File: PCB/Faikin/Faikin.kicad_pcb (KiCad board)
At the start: 2 copper layers, 70 x 70 mm, 31 parts, among them J1 1x5, J2 TC2030-USB-NL-DS, J3 Reset, Q1 BSS138PS, U3 MD8942, U4 ESP32-S3-MINI-1

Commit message: PCB Update
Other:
- board text removed: "TC2030"

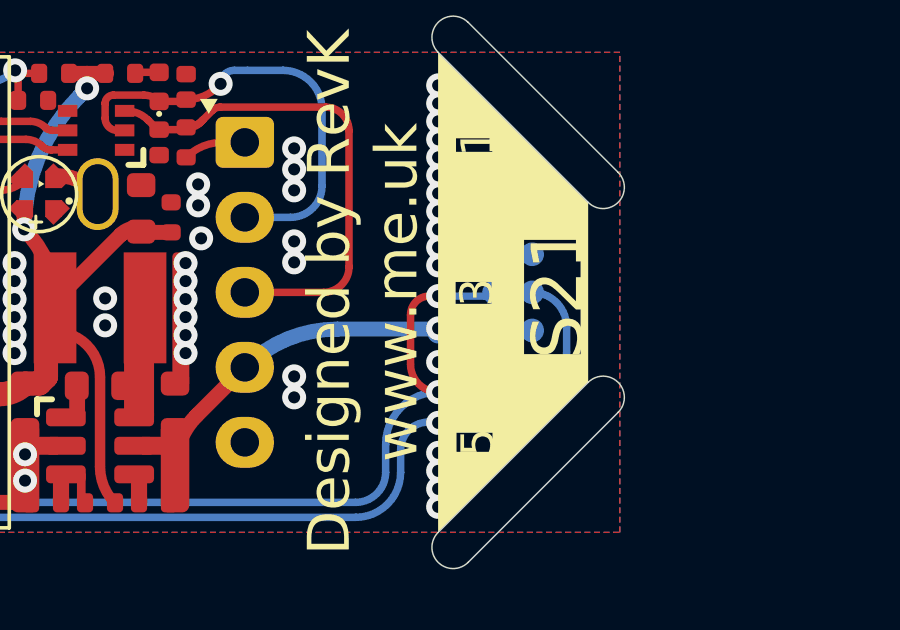
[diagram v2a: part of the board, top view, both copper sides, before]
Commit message: Library update
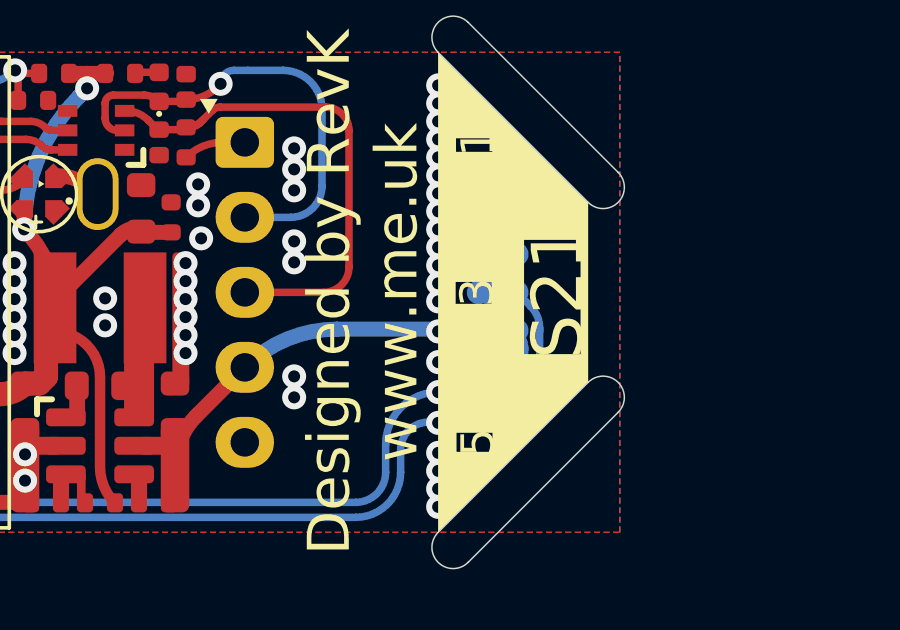
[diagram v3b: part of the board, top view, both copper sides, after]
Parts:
- moved J2 0.52 mm to (154.0, 65.0)
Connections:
- J2 pad 2: DC -> D-
- J2 pad 6: GND -> D-
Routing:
- net D-: track 36.1 -> 38.1 mm, vias 3 -> 2
- net DC: track 14.6 -> 12.7 mm
- net D+: track 39.6 -> 38.4 mm
- net GND: vias 54 -> 56
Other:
- board text added: "TC2030"
